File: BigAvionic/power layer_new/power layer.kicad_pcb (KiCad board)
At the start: 4 copper layers, 68 x 68 mm, 58 parts, among them J1 Conn_01x02, J2 USB_C_Receptacle_USB2.0_16P, J3 Conn_01x04, J4 Conn_01x04, J5 Conn_01x04, J6 Conn_01x04, Q1 AO3401A, Q2 AO3401A, U1 LD1117S33TR_SOT223, U2 LTC4412xS6

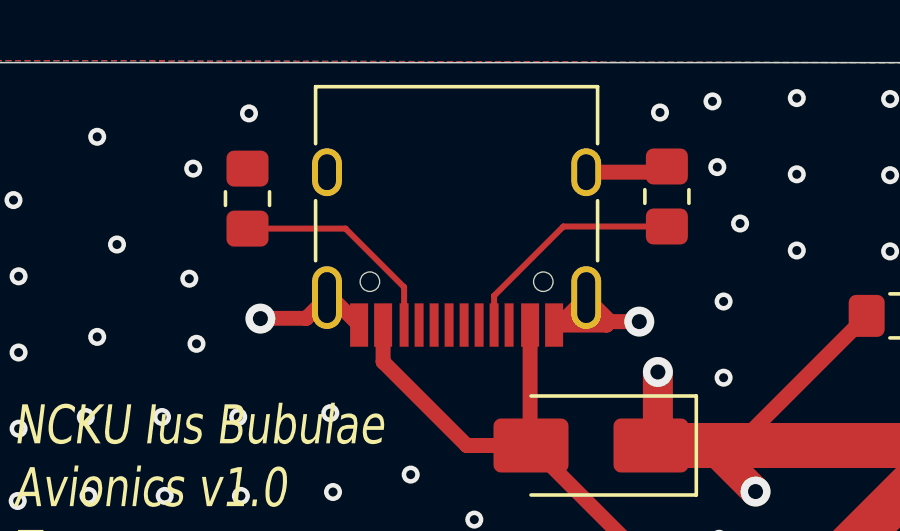
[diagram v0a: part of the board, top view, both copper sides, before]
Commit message: recommit production
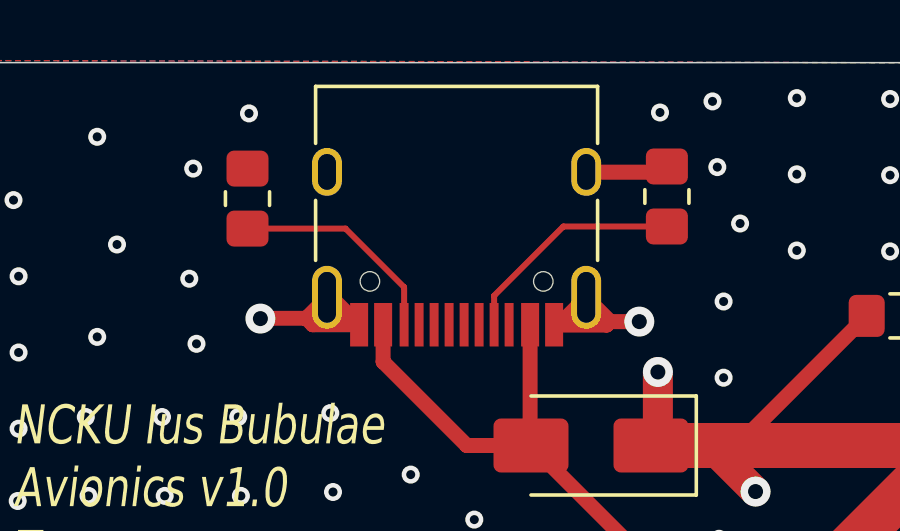
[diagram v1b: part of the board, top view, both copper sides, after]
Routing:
- net GND: track 73.7 -> 75.4 mm
